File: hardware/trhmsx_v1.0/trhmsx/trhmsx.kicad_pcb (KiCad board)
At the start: 2 copper layers, 170 x 170 mm, 123 parts, among them IC1 EPCS4, J1 MODULE-12V, J10 JOY2, J11 AudioJack2_Ground, J12 RCA, J13 CART2, J14 DH15, J15 JOY1, J16 CART1, J2 ESP-01, J3 Barrel_Jack, J4 MICRO-SD, J5 Conn_01x02, J6 KEYBOARD-USB, J7 KEYBOARD-PS2, J8 Conn_02x05_Odd_Even, J9 EXPANSION, SW1 SW_DIP_x08, SW2 SW_Push, U1 EP1C12Q240C8N, U2 AMS1117-1.5, U3 AMS1117-3.3, U4 NC7WZU04P6X, U5 MT48LC16M16A2TG, U6 M51953BFP, Y1 21.47727 MHz

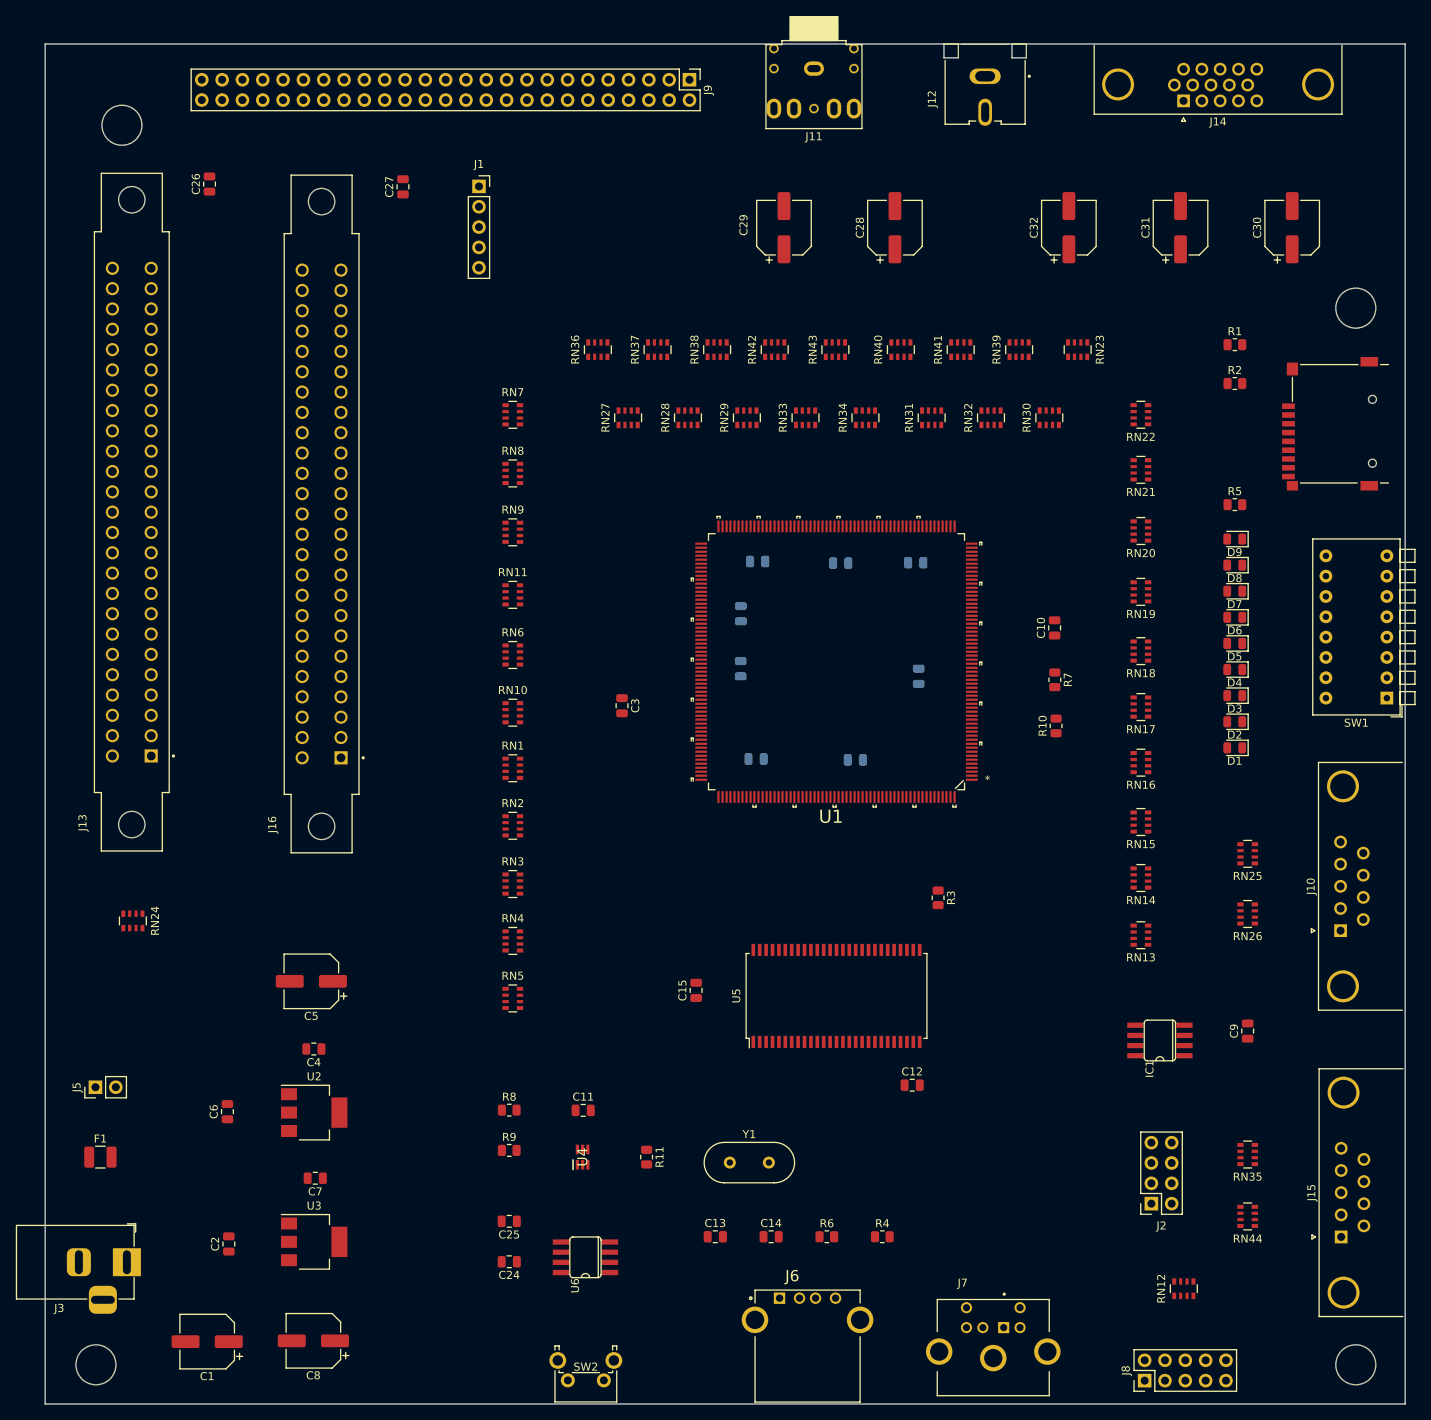
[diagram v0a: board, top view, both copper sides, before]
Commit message: Initial placement
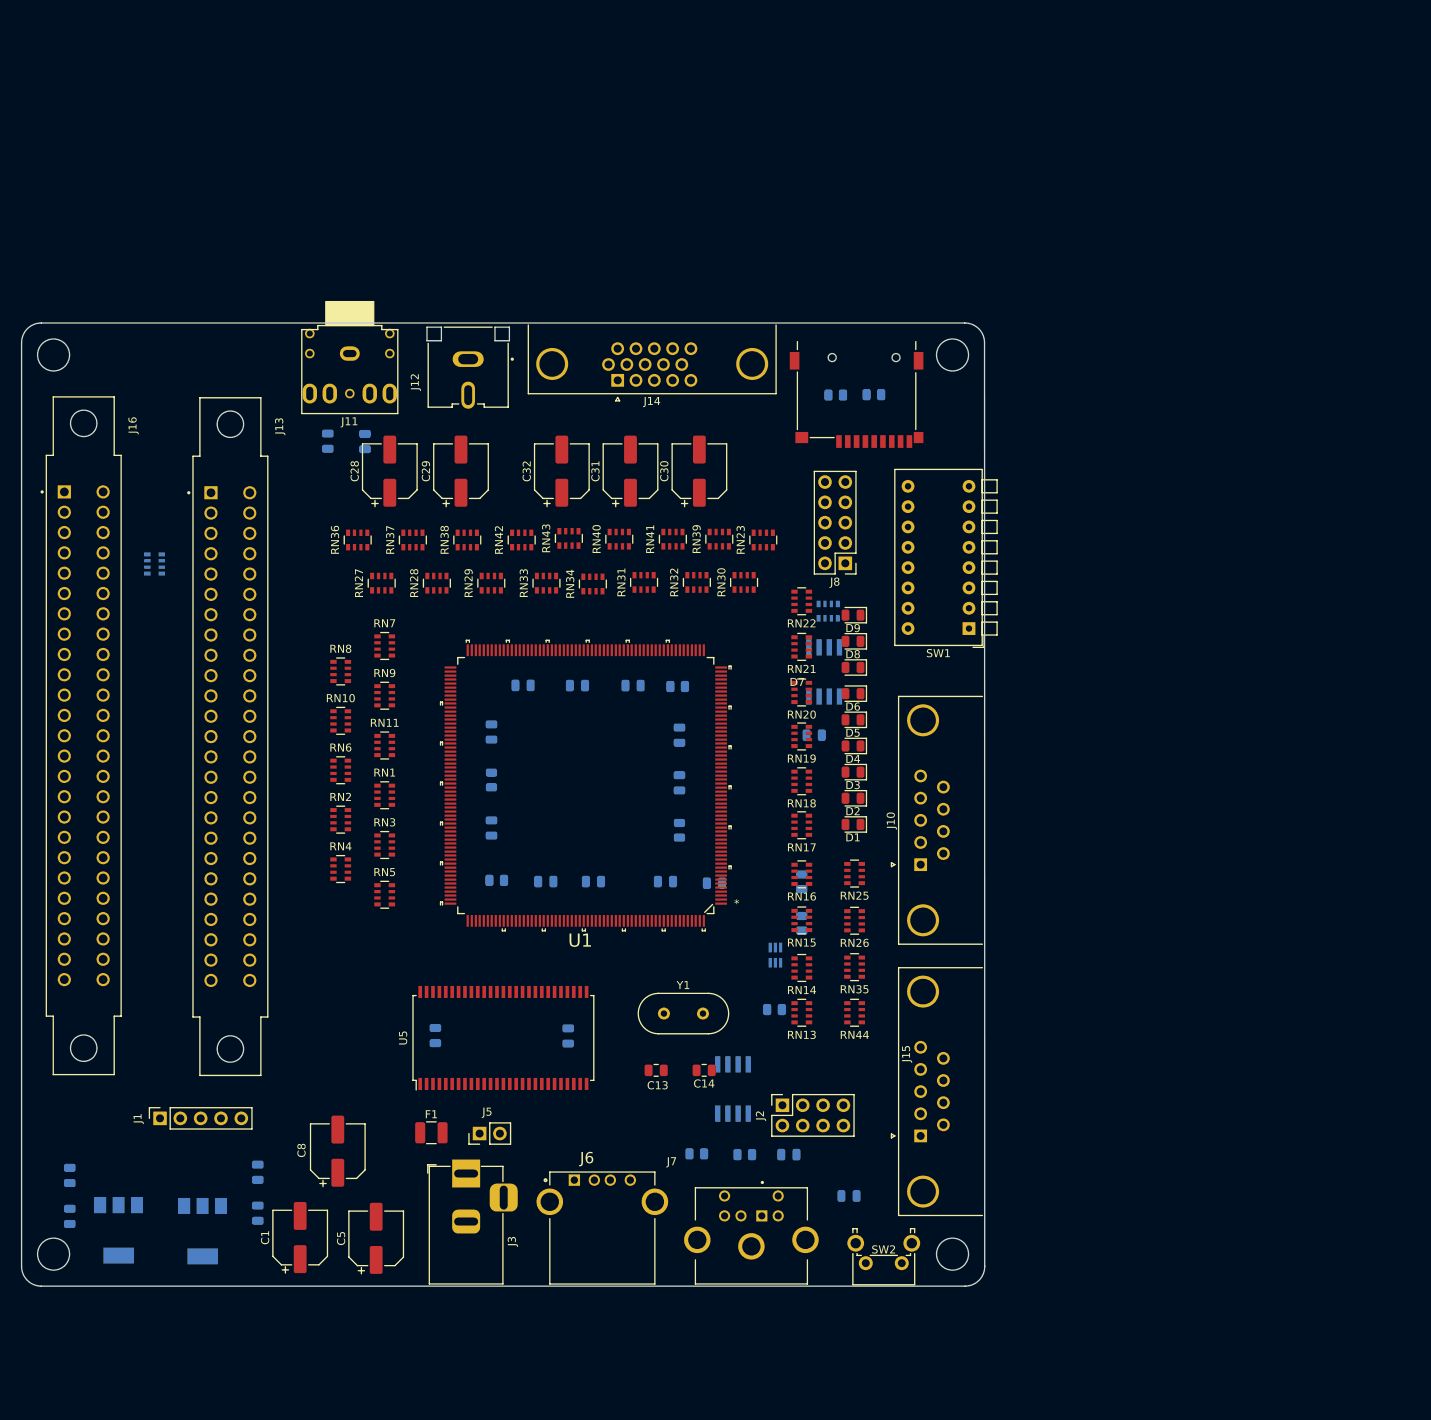
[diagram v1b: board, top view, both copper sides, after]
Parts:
- removed J9: EXPANSION, Connector_PinHeader_2.54mm:PinHeader_2x25_P2.54mm_Vertical
- C10, C11, C12, C15, C2, C24, C25, C26, C27, C3, C4, C6, C7, C9, IC1, R1, R10, R11, R2, R3, R4, R5, R6, R7, R8, R9, RN12, RN24, U2, U3, U4, U6: moved to B.Cu
- moved J1 123.1 mm to (145.8, 188.4), turned to 90 degrees
- moved J8 108.8 mm to (231.4, 119.0), turned to 180 degrees
- moved RN12 95.6 mm to (229.3, 125.0)
- moved C30 80.1 mm to (213.2, 107.5)
- moved J14 78.9 mm to (203.0, 96.2)
- moved C31 75.2 mm to (204.6, 107.5)
- moved J12 73.7 mm to (184.3, 93.5)
- moved R5 73.3 mm to (210.5, 134.4)
- moved R10 72.5 mm to (187.9, 158.6), turned to 0 degrees
- moved C32 70.3 mm to (196.0, 107.5)
- moved C28 70.1 mm to (174.5, 107.5)
- moved J11 68.1 mm to (169.5, 95.8)
- moved C9 65.6 mm to (227.6, 140.5), turned to 180 degrees
- moved J4 65.0 mm to (232.8, 93.3), turned to 180 degrees
- moved IC1 62.3 mm to (228.8, 132.6), turned to 180 degrees
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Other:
- board size 170 x 170 mm -> 120.4 x 120.4 mm
